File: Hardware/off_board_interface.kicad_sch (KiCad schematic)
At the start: 1 part, among them J2 GMI-10-2-1.27-G-10

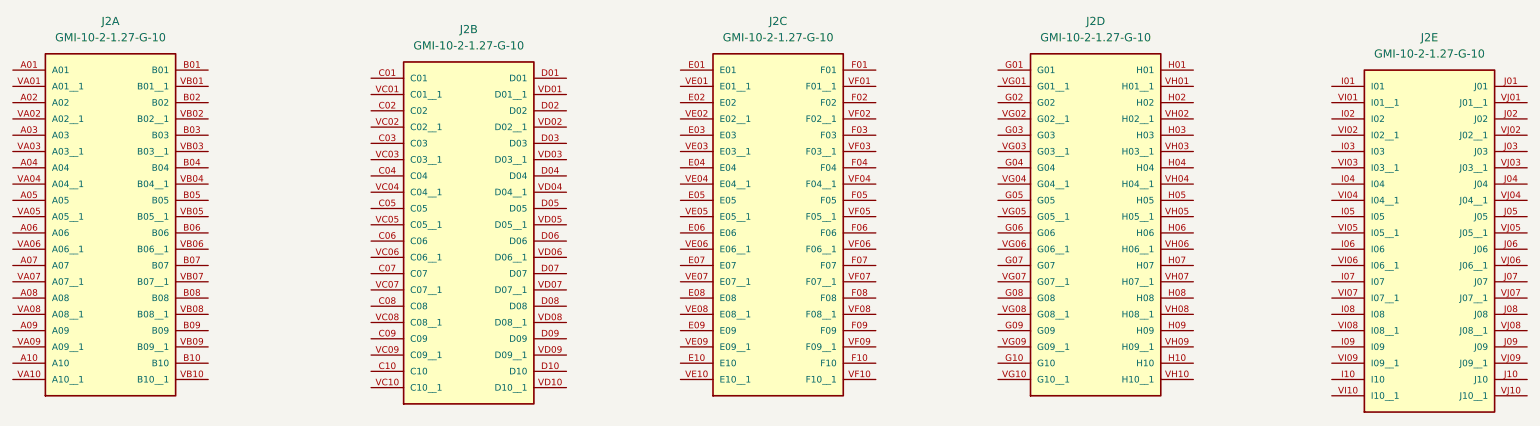
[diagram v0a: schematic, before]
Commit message: Trying to assign MGT lanes but I don't know how to do inter sheet connectivity yet
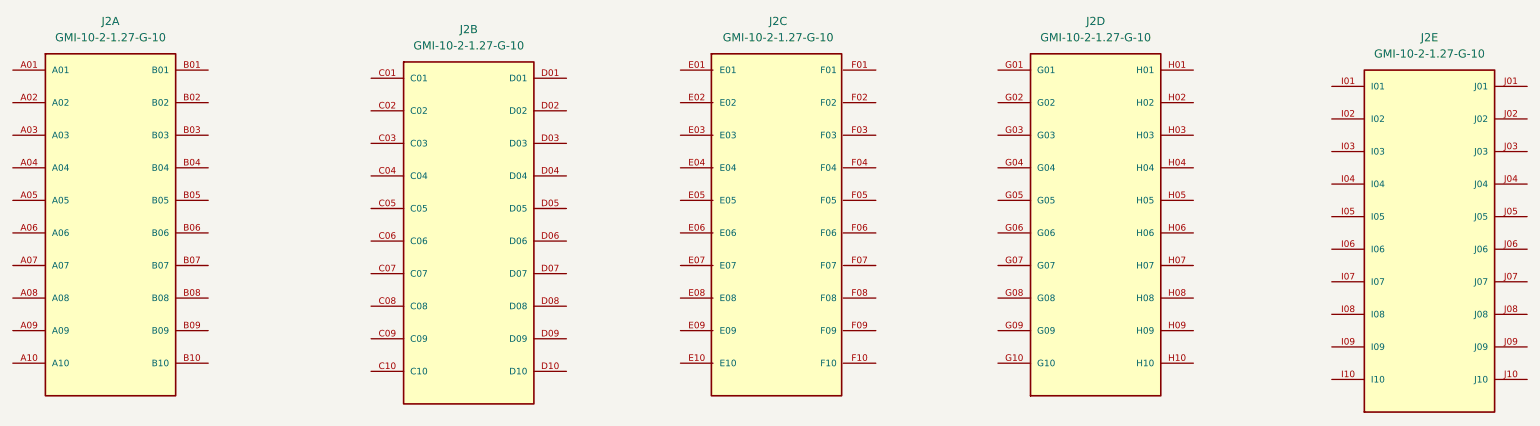
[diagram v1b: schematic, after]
